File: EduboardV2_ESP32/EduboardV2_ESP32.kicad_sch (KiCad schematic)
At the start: 1 part, among them U1 ESP32-WROOM-E

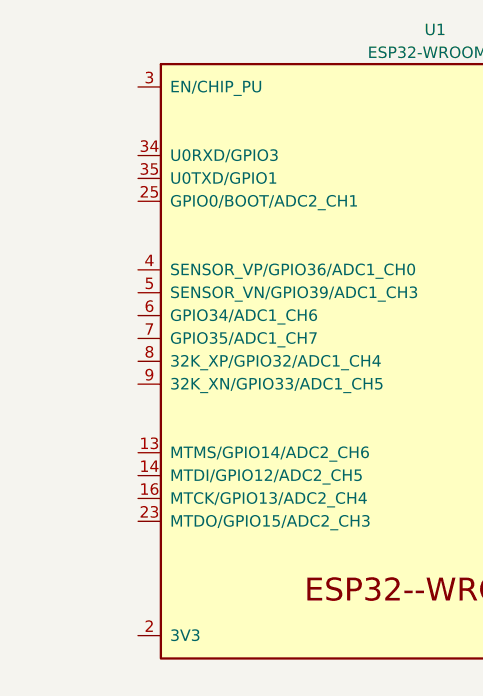
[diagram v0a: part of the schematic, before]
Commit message: work on debug chip
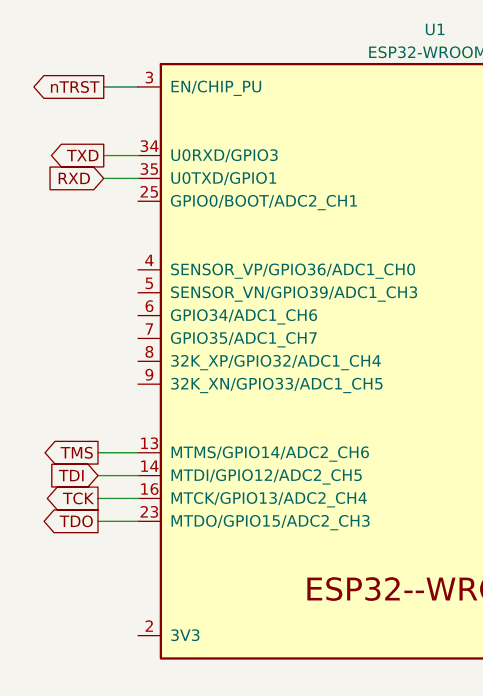
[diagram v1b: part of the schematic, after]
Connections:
- net TMS: now reaches U1.13 (MTMS/GPIO14/ADC2_CH6)
- net TDI: now reaches U1.14 (MTDI/GPIO12/ADC2_CH5)
- net TCK: now reaches U1.16 (MTCK/GPIO13/ADC2_CH4)
- net TDO: now reaches U1.23 (MTDO/GPIO15/ADC2_CH3)
- net nTRST: now reaches U1.3 (EN/CHIP_PU)
- net TXD: now reaches U1.34 (U0RXD/GPIO3)
- net RXD: now reaches U1.35 (U0TXD/GPIO1)
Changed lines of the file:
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@@
 (kicad_sch (version 20230121) (generator eeschema)
   (paper "A4")
+  (wire (pts (xy 74.295 46.99) (xy 78.105 46.99))
+    (stroke (width 0) (type default))
+  )
+  (wire (pts (xy 73.66 85.09) (xy 78.105 85.09))
+    (stroke (width 0) (type default))
+  )
+  (wire (pts (xy 73.66 82.55) (xy 78.105 82.55))
+    (stroke (width 0) (type default))
+  )
+  (wire (pts (xy 73.66 87.63) (xy 78.105 87.63))
+    (stroke (width 0) (type default))
+  )
+  (wire (pts (xy 74.295 39.37) (xy 78.105 39.37))
+    (stroke (width 0) (type default))
+  )
+  (wire (pts (xy 73.66 80.01) (xy 78.105 80.01))
+    (stroke (width 0) (type default))
+  )
+  (wire (pts (xy 74.295 49.53) (xy 78.105 49.53))
+    (stroke (width 0) (type default))
+  )
+  (global_label "RXD" (shape input) (at 74.295 49.53 180) (fields_autoplaced)
+    (effects (font (size 1.27 1.27)) (justify right))
+    (property "Intersheetrefs" "${INTERSHEET_REFS}" (at 67.6397 49.53 0)
+      (effects (font (size 1.27 1.27)) (justify right) hide)
+    )
+  )
+  (global_label "TCK" (shape output) (at 73.66 85.09 180) (fields_autoplaced)
+    (effects (font (size 1.27 1.27)) (justify right))
+    (property "Intersheetrefs" "${INTERSHEET_REFS}" (at 67.2466 85.09 0)
+      (effects (font (size 1.27 1.27)) (justify right) hide)
+    )
+  )
+  (global_label "TDI" (shape input) (at 73.66 82.55 180) (fields_autoplaced)
+    (effects (font (size 1.27 1.27)) (justify right))
+    (property "Intersheetrefs" "${INTERSHEET_REFS}" (at 67.9118 82.55 0)
+      (effects (font (size 1.27 1.27)) (justify right) hide)
+    )
+  )
+  (global_label "TMS" (shape output) (at 73.66 80.01 180) (fields_autoplaced)
+    (effects (font (size 1.27 1.27)) (justify right))
+    (property "Intersheetrefs" "${INTERSHEET_REFS}" (at 67.1257 80.01 0)
+      (effects (font (size 1.27 1.27)) (justify right) hide)
+    )
+  )
+  (global_label "TDO" (shape output) (at 73.66 87.63 180) (fields_autoplaced)
+    (effects (font (size 1.27 1.27)) (justify right))
+    (property "Intersheetrefs" "${INTERSHEET_REFS}" (at 67.1861 87.63 0)
+      (effects (font (size 1.27 1.27)) (justify right) hide)
+    )
+  )
+  (global_label "TXD" (shape output) (at 74.295 46.99 180) (fields_autoplaced)
+    (effects (font (size 1.27 1.27)) (justify right))
+    (property "Intersheetrefs" "${INTERSHEET_REFS}" (at 67.9421 46.99 0)
+      (effects (font (size 1.27 1.27)) (justify right) hide)
+    )
+  )
+  (global_label "nTRST" (shape output) (at 74.295 39.37 180) (fields_autoplaced)
+    (effects (font (size 1.27 1.27)) (justify right))
+    (property "Intersheetrefs" "${INTERSHEET_REFS}" (at 65.8255 39.37 0)
+      (effects (font (size 1.27 1.27)) (justify right) hide)
+    )
+  )
   (symbol (lib_id "Espressif:ESP32-WROOM-E") (at 111.125 69.85 0) (unit 1)
     (in_bom yes) (on_board yes) (dnp no) (fields_autoplaced)
